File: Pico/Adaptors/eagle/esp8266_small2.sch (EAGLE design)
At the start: 3 parts, among them U2 MCP1703T-3302E/CB

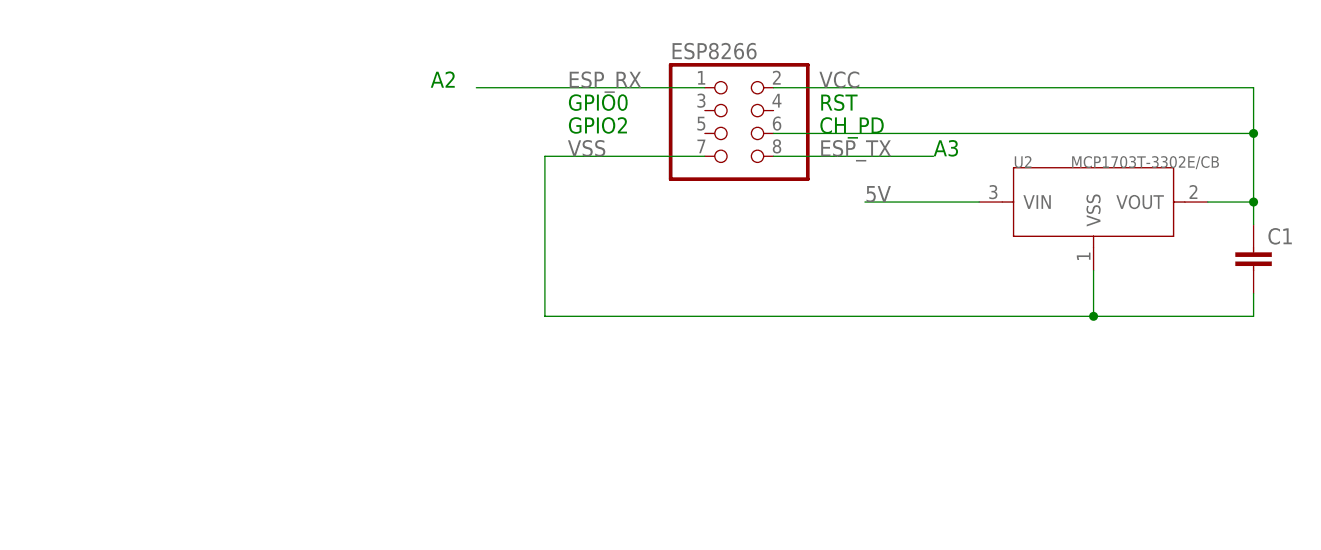
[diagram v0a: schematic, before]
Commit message: more tweaks and options
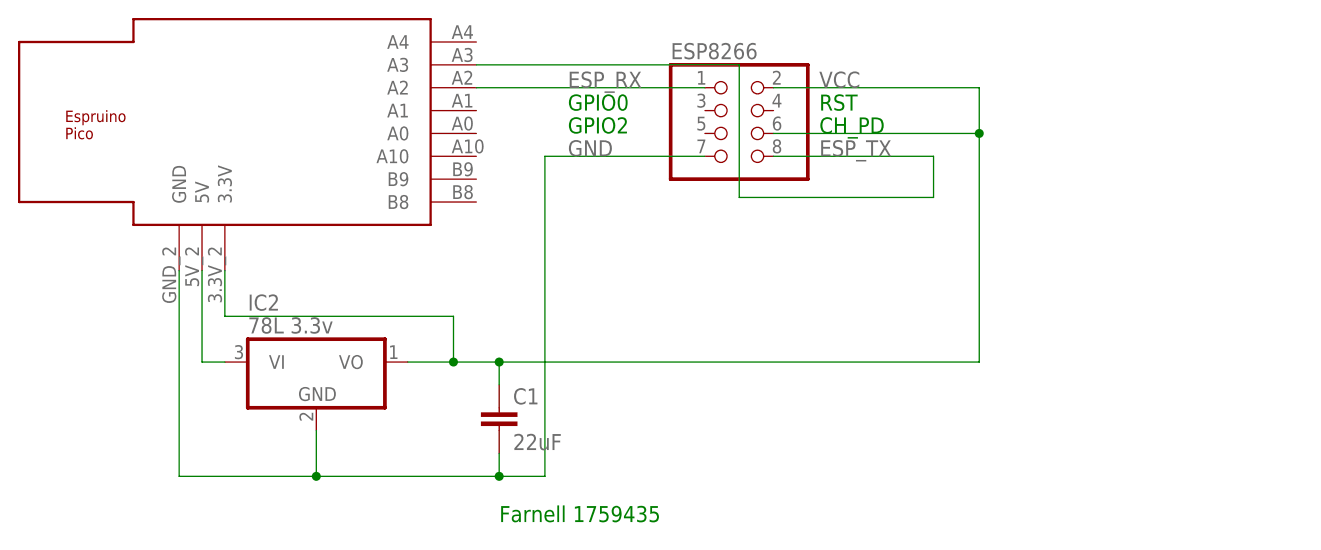
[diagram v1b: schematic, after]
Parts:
- removed U2: MCP1703T-3302E/CB, xc6206:XC6206
- added IC2: 78L 3.3v, linear:78L05Z
- added U$1: ESPRUINO_PICO_0.05, espruino_pico:ESPRUINO_PICO_0.05
- C1: value (none) -> 22uF; device rcl:C-EU025-050X050 -> rcl:C-EUC1210
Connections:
- removed net 5V: U2.VIN
- removed net VSS: C1.2, ESP8266.7, U2.VSS
- new net GND: C1.2, ESP8266.7, IC2.GND, U$1.GND
- new net N$1: IC2.VI, U$1.5V
- net ESP_RX: now also U$1.A2
- net ESP_TX: now also U$1.A3
- net VCC: now also IC2.VO, U$1.3.3V; no longer U2.VOUT
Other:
- note added: "Farnell 1759435"
- note removed: "A2"
- note removed: "A3"
- moved on the sheet: C1
